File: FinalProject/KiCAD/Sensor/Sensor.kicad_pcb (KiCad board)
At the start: 2 copper layers, 32.5 x 31 mm, 9 parts, among them J1 Battery, J2 Conn_01x02_Socket, J3 Conn_01x02_Socket, J4 Conn_01x02_Socket, U3 ADS1115IDGS

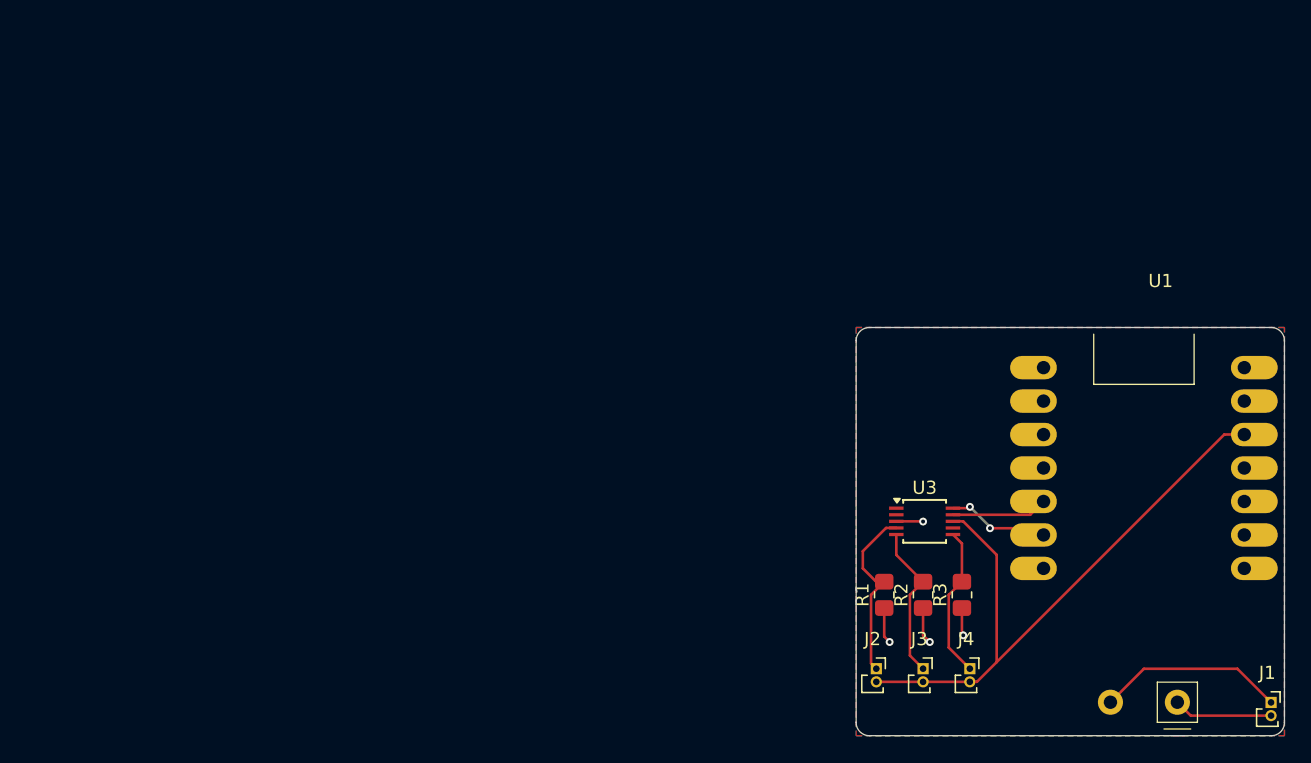
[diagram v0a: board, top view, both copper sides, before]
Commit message: Code
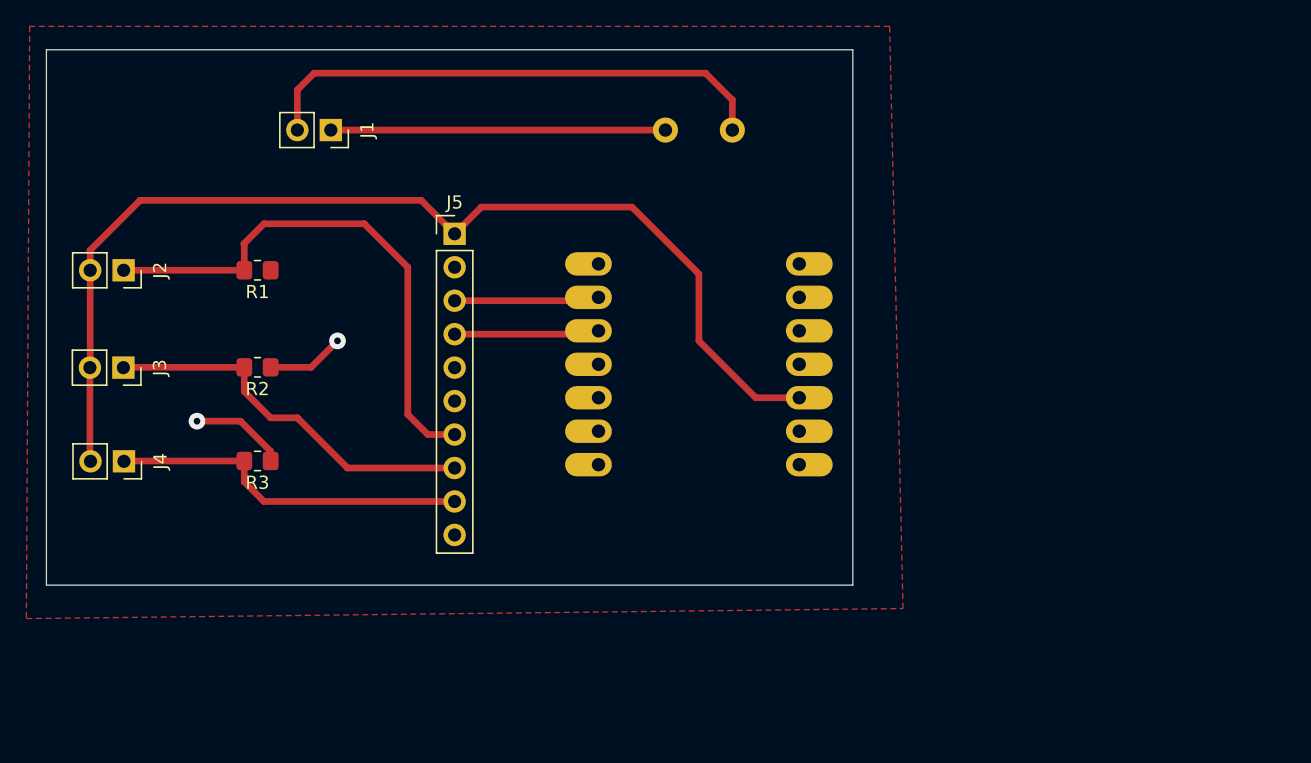
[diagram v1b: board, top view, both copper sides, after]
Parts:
- removed U3: ADS1115IDGS, Package_SO:TSSOP-10_3x3mm_P0.5mm
- added J5: Conn_01x10_Pin, Connector_PinHeader_2.54mm:PinHeader_1x10_P2.54mm_Vertical, F.Cu at (109.5, 72.4)
- J1, J2, J3, J4: footprint Connector_PinSocket_1.00mm:PinSocket_1x02_P1.00mm_Vertical -> Connector_PinSocket_2.54mm:PinSocket_1x02_P2.54mm_Vertical
- U1: moved to B.Cu
- moved J1 83.6 mm to (100.1, 64.5), turned to -90 degrees
- moved J4 66.1 mm to (84.4, 89.7), turned to -90 degrees
- moved J3 64.9 mm to (84.3, 82.5), turned to -90 degrees
- moved J2 64.6 mm to (84.3, 75.2), turned to -90 degrees
- moved R3 54.4 mm to (94.5, 89.6), turned to 180 degrees
- moved R1 53.6 mm to (94.5, 75.2), turned to 180 degrees
- moved R2 53.4 mm to (94.5, 82.5), turned to 180 degrees
- moved U1 34.7 mm to (128.0, 82.3)
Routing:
- net +3V3: track 48.2 -> 82.3 mm
- net -BATT: track 7.53 -> 39.7 mm
- net Net-(J2-Pin_1): track 13.8 -> 41.0 mm
- net Net-(J3-Pin_1): track 11.9 -> 29.4 mm
- net Net-(J4-Pin_1): track 11.5 -> 27.3 mm
- net +BATT: track 14.3 -> 25.4 mm
- net GND: track 9.69 -> 13.5 mm, vias 4 -> 2
- net /SDA: track 7.29 -> 11.0 mm
- net /SCL: track 7.86 -> 11.0 mm, vias 2 -> 0
- removed copper zone on B.Cu, net GND
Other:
- board size 32.5 x 31 mm -> 61.2 x 40.6 mm
